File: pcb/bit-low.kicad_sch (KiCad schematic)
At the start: 6 parts, among them Q222 2N7002K, Q223 2N7002K, Q224 2N7002K

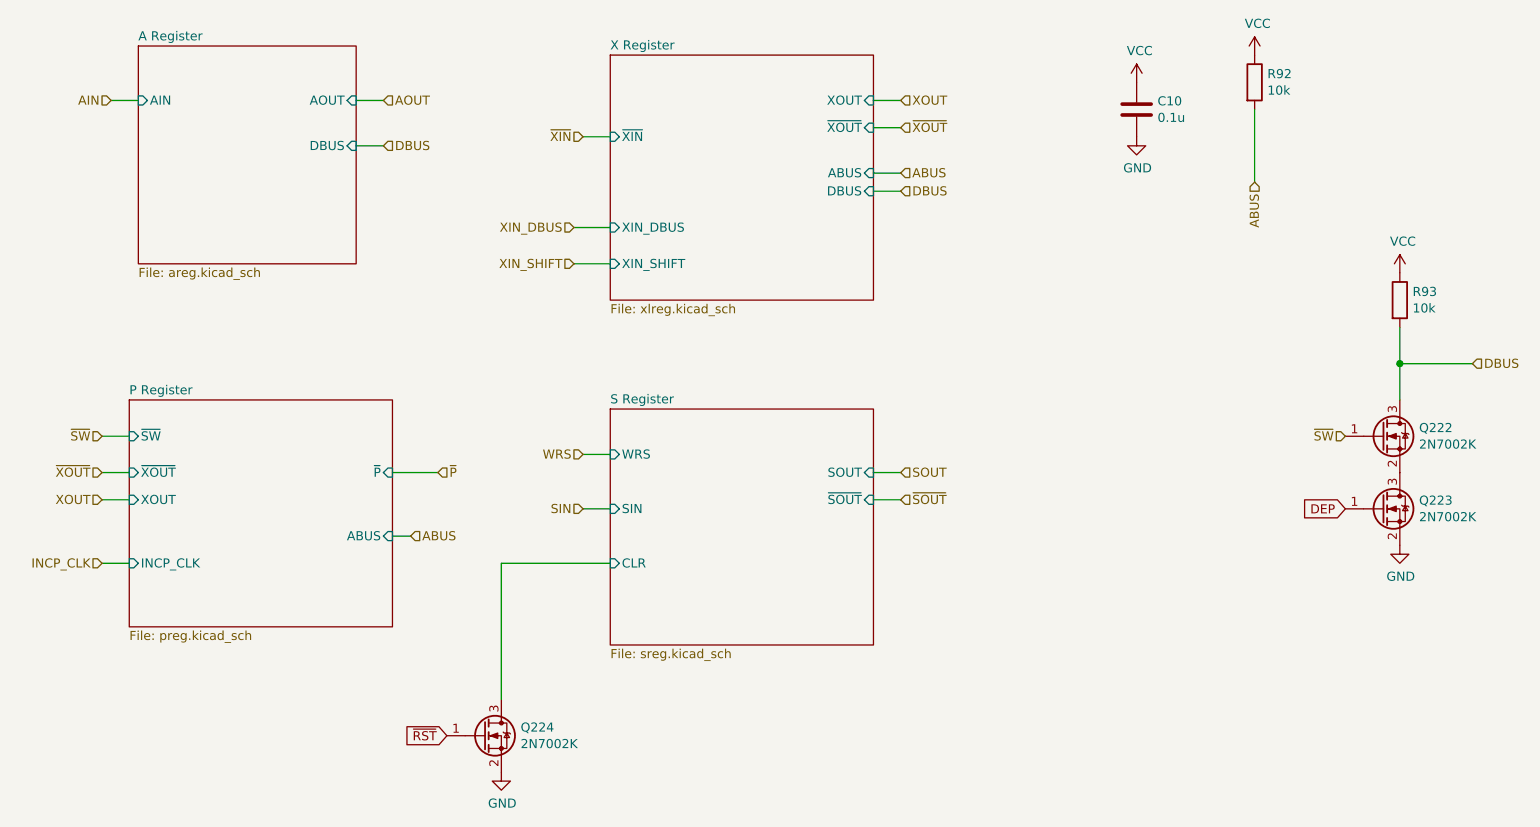
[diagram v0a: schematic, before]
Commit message: Revision 3.
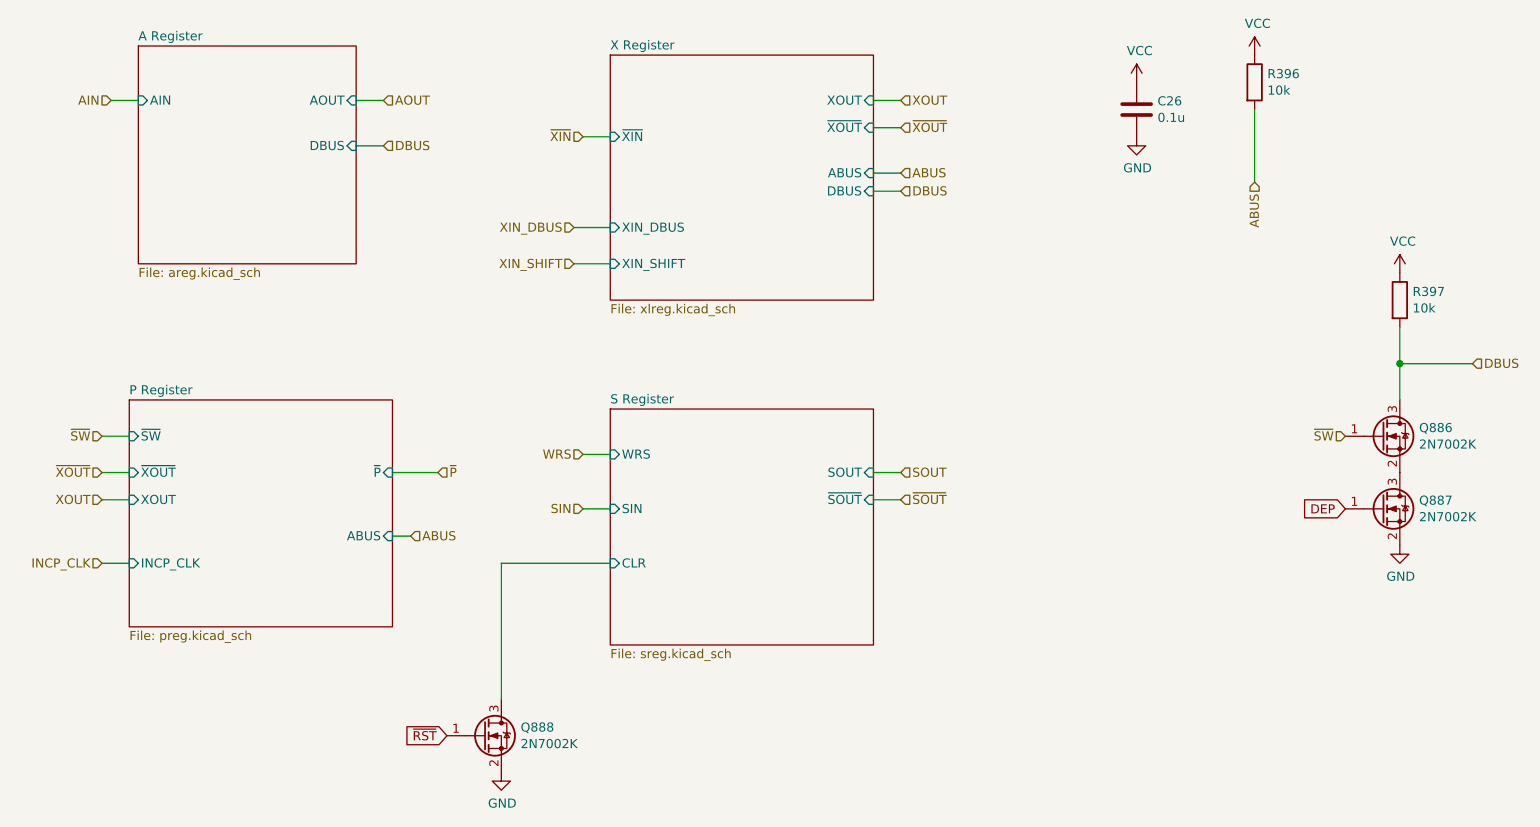
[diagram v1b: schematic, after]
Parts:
- renumbered C10 to C26, Q222 to Q886, Q223 to Q887, Q224 to Q888, R92 to R396, R93 to R397
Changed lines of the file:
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@@
   (symbol (lib_id "Device:R") (at 200.66 44.45 0)
     (in_bom yes) (on_board yes)
-    (property "Reference" "R92" (id 0) (at 202.438 43.2816 0)
+    (property "Reference" "R396" (id 0) (at 202.438 43.2816 0)
       (effects (font (size 1.27 1.27)) (justify left))
     )
@@
   (symbol (lib_id "Device:R") (at 220.98 74.93 0)
     (in_bom yes) (on_board yes)
-    (property "Reference" "R93" (id 0) (at 222.758 73.7616 0)
+    (property "Reference" "R397" (id 0) (at 222.758 73.7616 0)
       (effects (font (size 1.27 1.27)) (justify left))
     )
@@
   (symbol (lib_id "Device:C") (at 184.15 48.26 0)
     (in_bom yes) (on_board yes)
-    (property "Reference" "C10" (id 0) (at 187.071 47.0916 0)
+    (property "Reference" "C26" (id 0) (at 187.071 47.0916 0)
       (effects (font (size 1.27 1.27)) (justify left))
     )
@@
   (symbol (lib_id "Transistor_FET:2N7002") (at 92.71 135.89 0)
     (in_bom yes) (on_board yes)
-    (property "Reference" "Q224" (id 0) (at 97.9424 134.7216 0)
+    (property "Reference" "Q888" (id 0) (at 97.9424 134.7216 0)
       (effects (font (size 1.27 1.27)) (justify left))
     )
@@
   (symbol (lib_id "Transistor_FET:2N7002") (at 218.44 93.98 0)
     (in_bom yes) (on_board yes)
-    (property "Reference" "Q222" (id 0) (at 223.6724 92.8116 0)
+    (property "Reference" "Q886" (id 0) (at 223.6724 92.8116 0)
       (effects (font (size 1.27 1.27)) (justify left))
     )
@@
   (symbol (lib_id "Transistor_FET:2N7002") (at 218.44 104.14 0)
     (in_bom yes) (on_board yes)
-    (property "Reference" "Q223" (id 0) (at 223.6724 102.9716 0)
+    (property "Reference" "Q887" (id 0) (at 223.6724 102.9716 0)
       (effects (font (size 1.27 1.27)) (justify left))
     )
